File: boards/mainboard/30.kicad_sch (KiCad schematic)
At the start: 9 parts, among them U30 74163, U31 74163, U32 74163, U33 7400, U34 7474, U62 7486

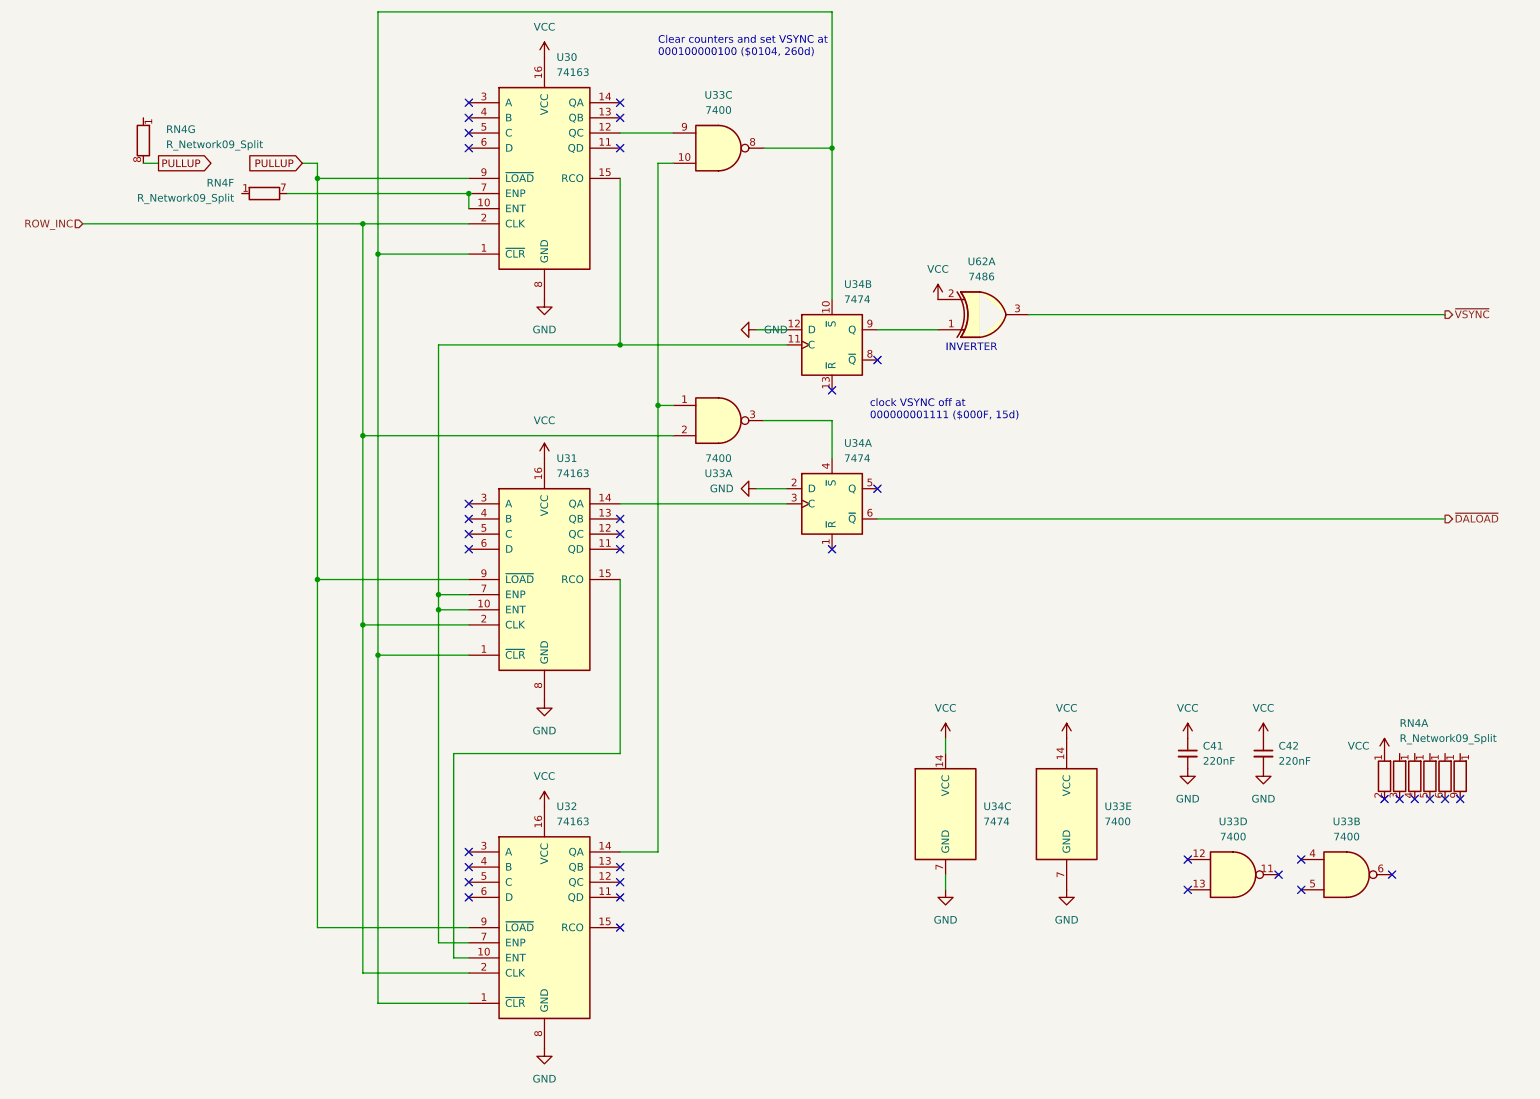
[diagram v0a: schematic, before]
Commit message: organize mainboard schematic
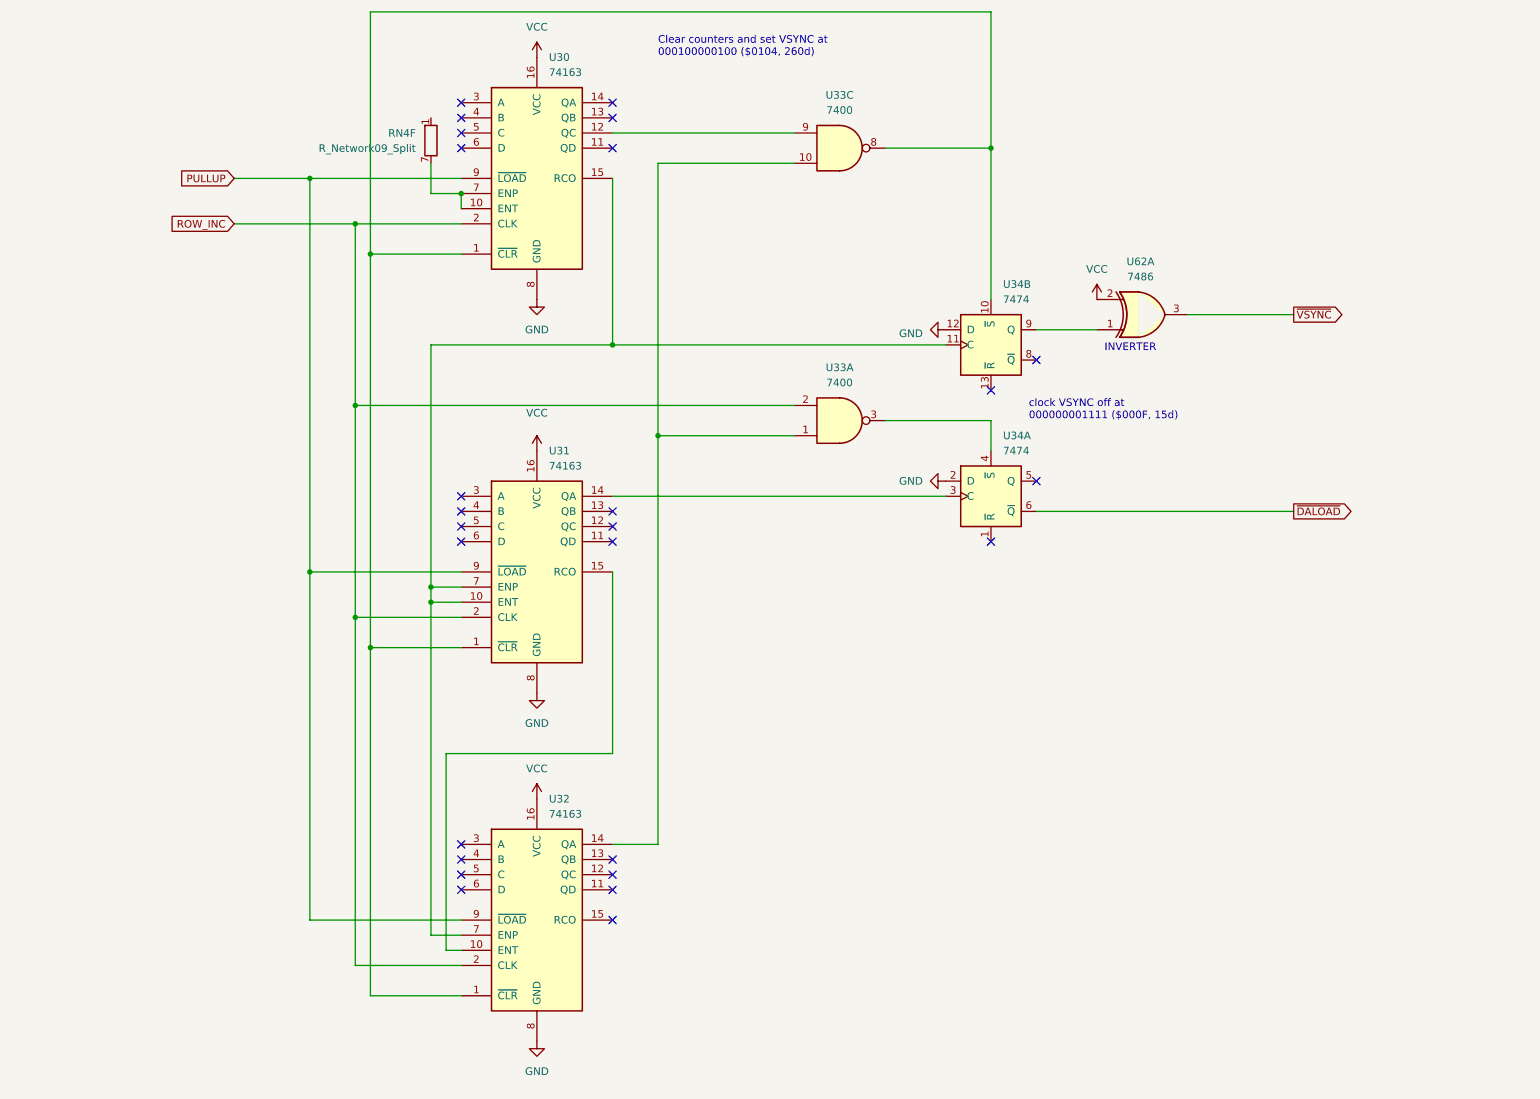
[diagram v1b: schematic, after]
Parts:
- removed C41, C42: 220nF, ambassador:C_Disc_D4.3mm_W1.9mm_P6.35mm, symbol Device:C_Small
- removed unit 1 of RN4
- removed unit 8 of RN4
- removed unit 5 of RN4
- removed unit 4 of RN4
- removed unit 7 of RN4
- removed unit 2 of RN4
- removed unit 3 of RN4
- removed unit 4 of U33
- removed unit 2 of U33
- removed unit 5 of U33
- removed unit 3 of U34
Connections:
- no-connect marks 38 -> 26
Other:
- moved on the sheet: RN4F, U30, U31, U32, U33A, U33C, U34A, U34B, U62A
